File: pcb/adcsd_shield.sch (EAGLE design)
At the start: 20 parts, among them X1 MCP3208

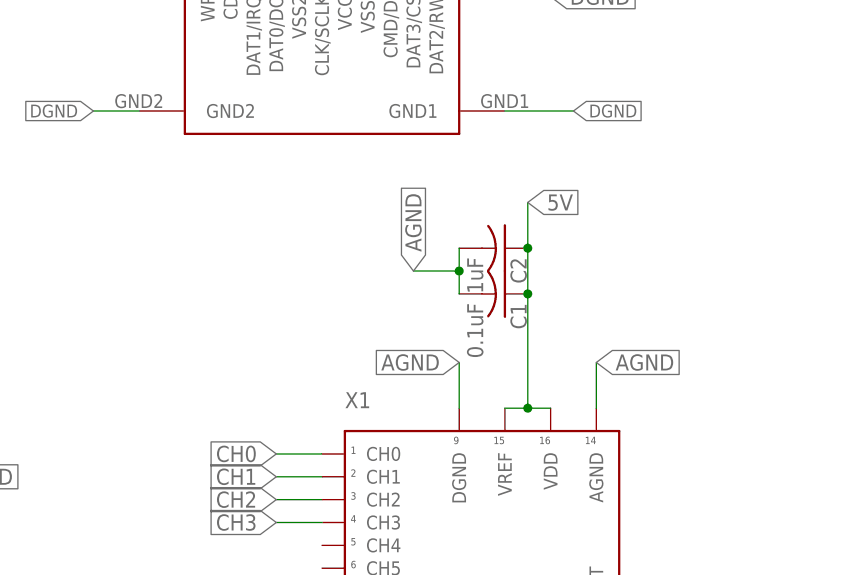
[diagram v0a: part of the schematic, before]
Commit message: some circuit modifications, updates
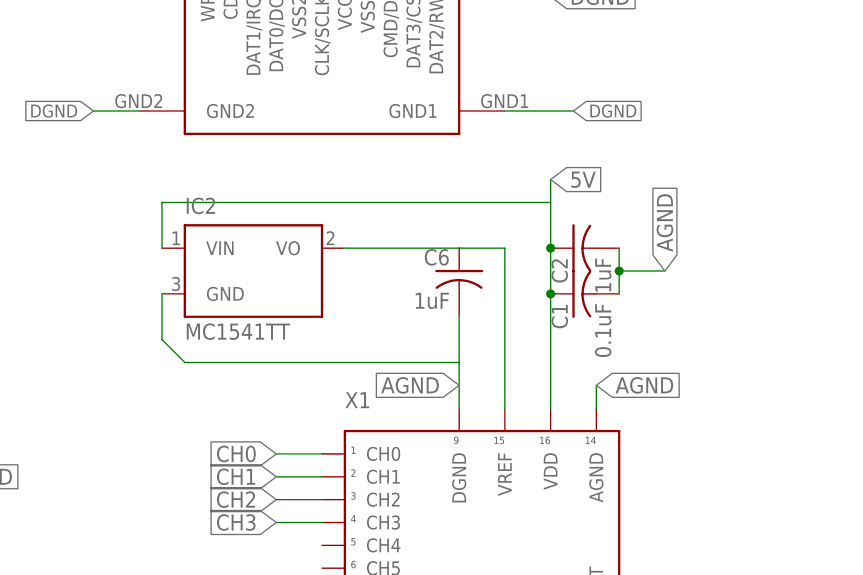
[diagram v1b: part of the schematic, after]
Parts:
- added C6: 1uF, rcl:C-USC0402
- added IC2: MC1541TT, microchip:MC1541TT
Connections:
- new net N$9: C6.1, IC2.VO, X1.VREF
- net 5V: now also IC2.VIN; no longer X1.VREF
- net AGND: now also C6.2, IC2.GND
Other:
- moved on the sheet: C1, C2
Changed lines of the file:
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@@
 <?xml version="1.0" encoding="utf-8"?>
 <!DOCTYPE eagle SYSTEM "eagle.dtd">
-<eagle version="6.6.0">
+<eagle version="7.3.0">
 <drawing>
 <settings>
@@
 <part name="C5" library="rcl" deviceset="C-US" device="C0402" value="1uF"/>
 <part name="SL1" library="con-lsta" deviceset="FE05-1" device=""/>
+<part name="IC2" library="microchip" deviceset="MC15*" device="TT" technology="41"/>
+<part name="C6" library="rcl" deviceset="C-US" device="C0402" value="1uF"/>
 </parts>
 <sheets>
@@
 <instance part="SV3" gate="G$1" x="-22.86" y="96.52"/>
 <instance part="SV1" gate="1" x="-22.86" y="139.7" rot="R180"/>
-<instance part="C1" gate="G$1" x="55.88" y="91.44" rot="R270"/>
-<instance part="C2" gate="G$1" x="55.88" y="96.52" rot="R270"/>
+<instance part="C1" gate="G$1" x="63.5" y="91.44" rot="MR270"/>
+<instance part="C2" gate="G$1" x="63.5" y="96.52" rot="MR270"/>
 <instance part="C5" gate="G$1" x="60.96" y="132.08"/>
 <instance part="SL1" gate="G$1" x="-20.32" y="50.8"/>
+<instance part="IC2" gate="G$1" x="27.94" y="93.98"/>
+<instance part="C6" gate="G$1" x="50.8" y="93.98" rot="MR0"/>
 </instances>
 <busses>
@@
 <segment>
 <pinref part="X1" gate="G$1" pin="VDD"/>
-<pinref part="X1" gate="G$1" pin="VREF"/>
-<wire x1="55.88" y1="78.74" x2="58.42" y2="78.74" width="0.1524" layer="91"/>
-<wire x1="58.42" y1="78.74" x2="60.96" y2="78.74" width="0.1524" layer="91"/>
-<wire x1="58.42" y1="78.74" x2="58.42" y2="91.44" width="0.1524" layer="91"/>
-<label x="58.42" y="101.6" size="1.778" layer="95" xref="yes"/>
+<wire x1="60.96" y1="78.74" x2="60.96" y2="91.44" width="0.1524" layer="91"/>
+<label x="60.96" y="104.14" size="1.778" layer="95" xref="yes"/>
 <pinref part="C2" gate="G$1" pin="1"/>
-<junction x="58.42" y="96.52"/>
-<wire x1="58.42" y1="91.44" x2="58.42" y2="96.52" width="0.1524" layer="91"/>
-<wire x1="58.42" y1="96.52" x2="58.42" y2="101.6" width="0.1524" layer="91"/>
+<junction x="60.96" y="96.52"/>
+<wire x1="60.96" y1="91.44" x2="60.96" y2="96.52" width="0.1524" layer="91"/>
+<wire x1="60.96" y1="96.52" x2="60.96" y2="101.6" width="0.1524" layer="91"/>
 <pinref part="C1" gate="G$1" pin="1"/>
-<junction x="58.42" y="91.44"/>
-<junction x="58.42" y="78.74"/>
+<junction x="60.96" y="91.44"/>
+<pinref part="IC2" gate="G$1" pin="VIN"/>
+<wire x1="60.96" y1="101.6" x2="60.96" y2="104.14" width="0.1524" layer="91"/>
+<wire x1="60.96" y1="101.6" x2="17.78" y2="101.6" width="0.1524" layer="91"/>
+<wire x1="17.78" y1="101.6" x2="17.78" y2="96.52" width="0.1524" layer="91"/>
 </segment>
 <segment>
@@
 <segment>
 <pinref part="X1" gate="G$1" pin="DGND"/>
+<label x="50.8" y="81.28" size="1.778" layer="95" rot="R180" xref="yes"/>
+<pinref part="C6" gate="G$1" pin="2"/>
+<wire x1="50.8" y1="88.9" x2="50.8" y2="83.82" width="0.1524" layer="91"/>
+<pinref part="IC2" gate="G$1" pin="GND"/>
 <wire x1="50.8" y1="83.82" x2="50.8" y2="78.74" width="0.1524" layer="91"/>
-<label x="50.8" y="83.82" size="1.778" layer="95" rot="R180" xref="yes"/>
+<wire x1="17.78" y1="91.44" x2="17.78" y2="86.36" width="0.1524" layer="91"/>
+<wire x1="17.78" y1="86.36" x2="20.32" y2="83.82" width="0.1524" layer="91"/>
+<wire x1="20.32" y1="83.82" x2="50.8" y2="83.82" width="0.1524" layer="91"/>
 </segment>
 <segment>
 <pinref part="X1" gate="G$1" pin="AGND"/>
-<wire x1="66.04" y1="83.82" x2="66.04" y2="78.74" width="0.1524" layer="91"/>
-<label x="66.04" y="83.82" size="1.778" layer="95" xref="yes"/>
+<wire x1="66.04" y1="81.28" x2="66.04" y2="78.74" width="0.1524" layer="91"/>
+<label x="66.04" y="81.28" size="1.778" layer="95" xref="yes"/>
 </segment>
 <segment>
@@
 <pinref part="C2" gate="G$1" pin="2"/>
 <pinref part="C1" gate="G$1" pin="2"/>
-<wire x1="50.8" y1="96.52" x2="50.8" y2="93.98" width="0.1524" layer="91"/>
-<wire x1="50.8" y1="93.98" x2="50.8" y2="91.44" width="0.1524" layer="91"/>
-<wire x1="50.8" y1="93.98" x2="45.72" y2="93.98" width="0.1524" layer="91"/>
-<label x="45.72" y="93.98" size="1.778" layer="95" rot="R90" xref="yes"/>
-<junction x="50.8" y="93.98"/>
+<wire x1="68.58" y1="96.52" x2="68.58" y2="93.98" width="0.1524" layer="91"/>
+<wire x1="68.58" y1="93.98" x2="68.58" y2="91.44" width="0.1524" layer="91"/>
+<wire x1="68.58" y1="93.98" x2="73.66" y2="93.98" width="0.1524" layer="91"/>
+<label x="73.66" y="93.98" size="1.778" layer="95" rot="R90" xref="yes"/>
+<junction x="68.58" y="93.98"/>
 </segment>
 </net>
@@
 </segment>
 </net>
+<net name="N$9" class="0">
+<segment>
+<pinref part="IC2" gate="G$1" pin="VO"/>
+<pinref part="C6" gate="G$1" pin="1"/>
+<wire x1="38.1" y1="96.52" x2="50.8" y2="96.52" width="0.1524" layer="91"/>
+<wire x1="50.8" y1="96.52" x2="55.88" y2="96.52" width="0.1524" layer="91"/>
+<pinref part="X1" gate="G$1" pin="VREF"/>
+<wire x1="55.88" y1="96.52" x2="55.88" y2="78.74" width="0.1524" layer="91"/>
+</segment>
+</net>
